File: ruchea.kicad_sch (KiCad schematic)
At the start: 10 parts, among them J14 Conn_01x03, J3 Conn_01x03, J4 Conn_01x04, J5 Conn_01x04, J6 Conn_01x02, J7 Conn_01x02, J8 Conn_01x03, J9 Conn_01x03

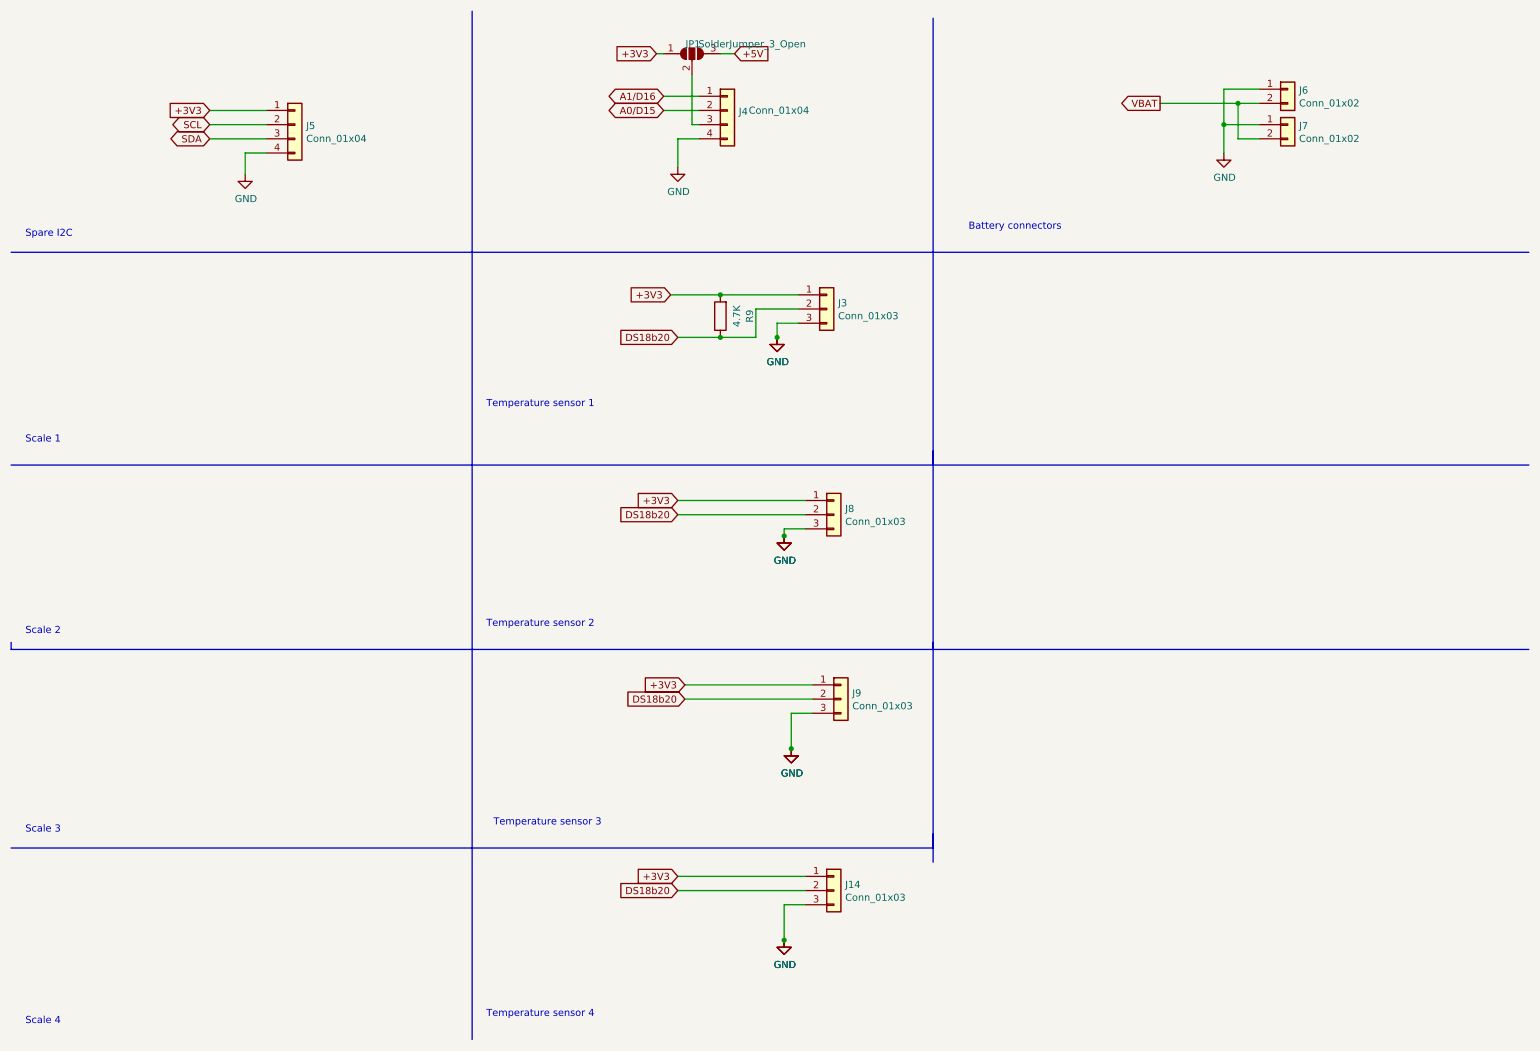
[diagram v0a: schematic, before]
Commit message: update
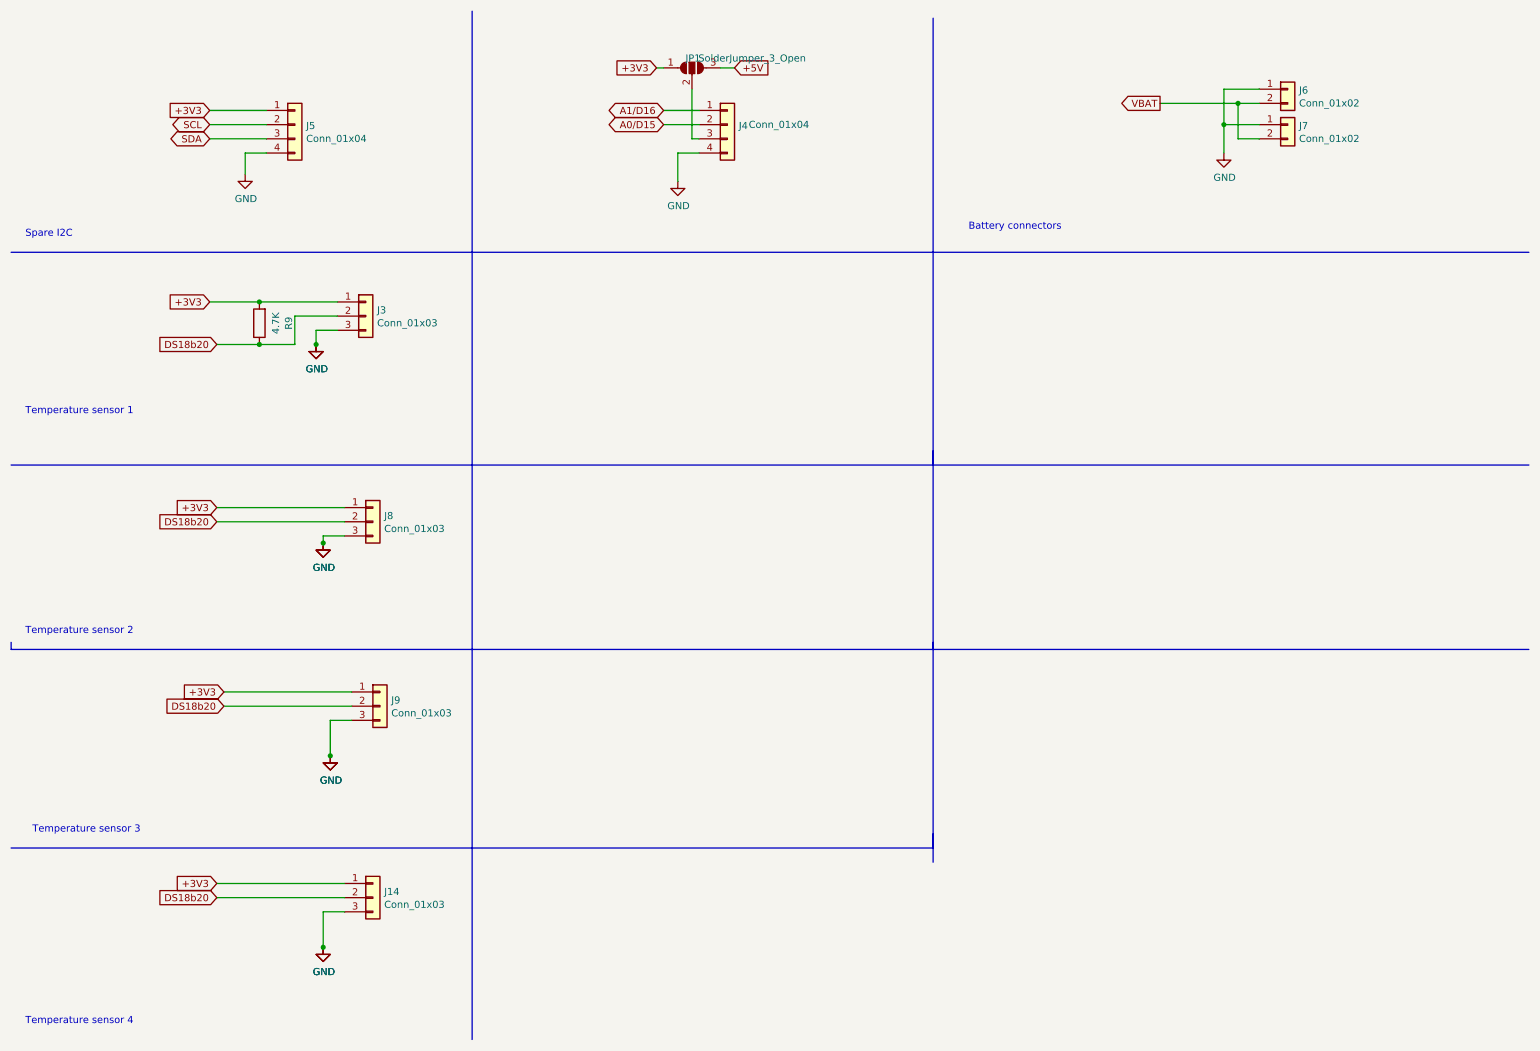
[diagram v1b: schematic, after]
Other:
- note removed: "Scale 1"
- note removed: "Scale 2"
- note removed: "Scale 3"
- note removed: "Scale 4"
- moved on the sheet: J14, J3, J4, J8, J9, JP1, R9
